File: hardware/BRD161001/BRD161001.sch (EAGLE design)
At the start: 42 parts, among them CN1 XH, CN2 JST XH, CN3 30306-6002HB, Q1 FDV301, Q2 DMP2035, Q3 FDV301, Q4 FDV301, U1 ATTINY44A-SSU, U2 TC4427AEOA, U3 TC4427AEOA, X1 32K768

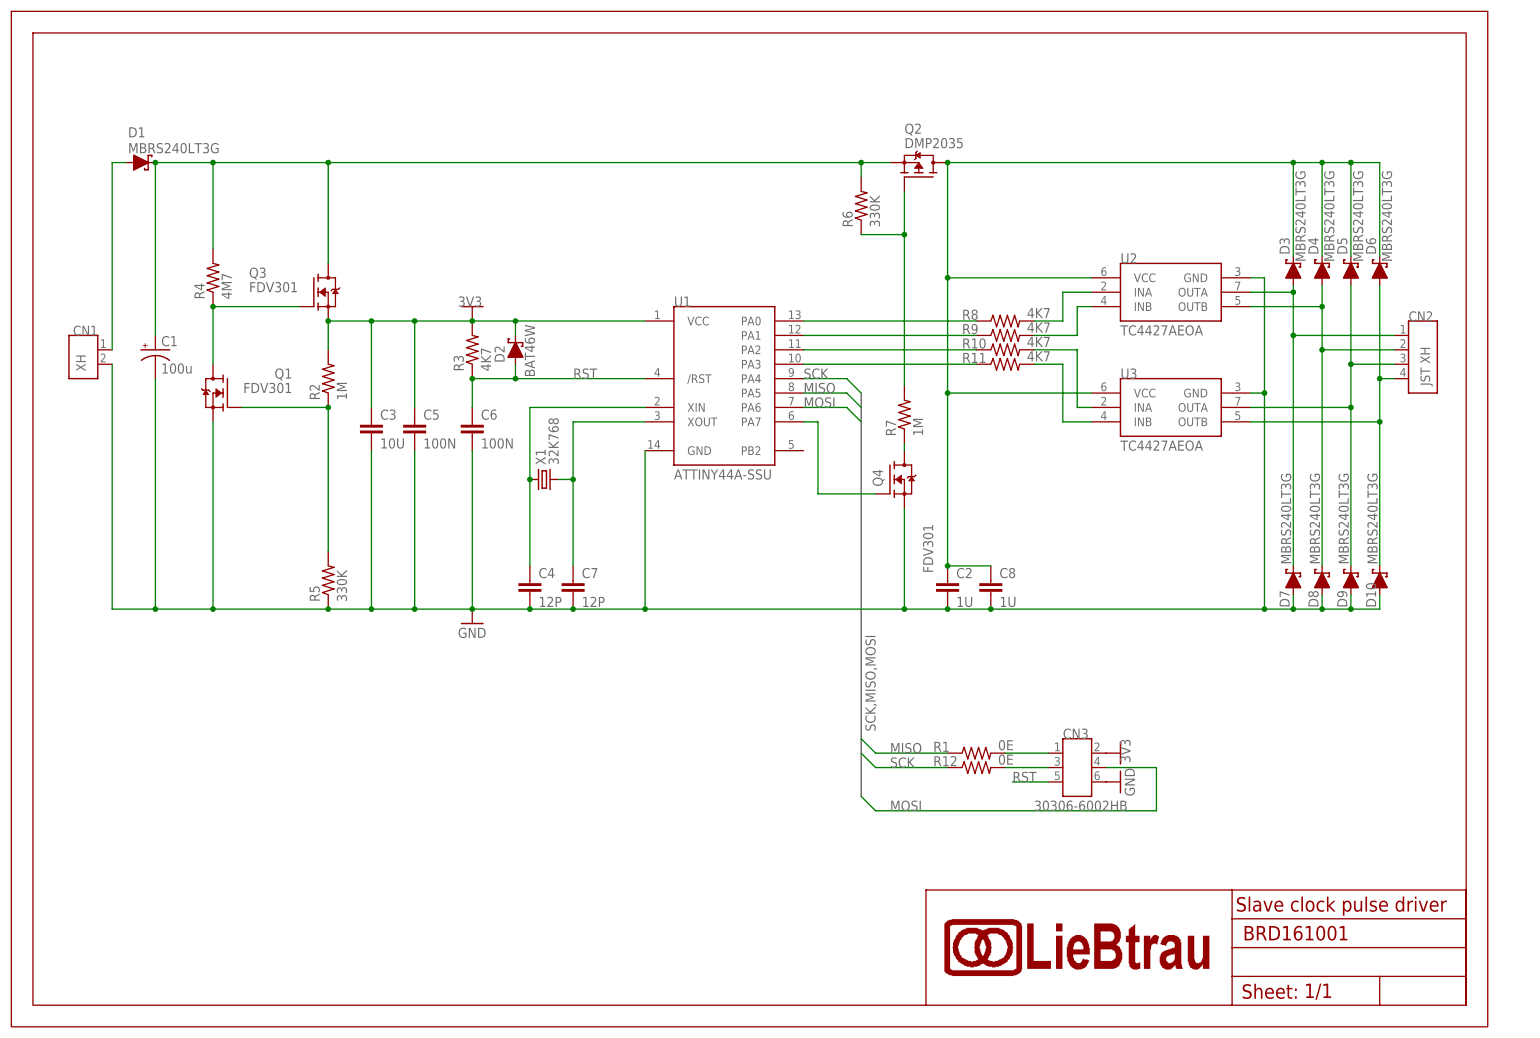
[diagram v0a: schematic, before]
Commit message: R1 of the hardware design
Signed-off-by: Christoph Tack <prog.send@gmail.com>
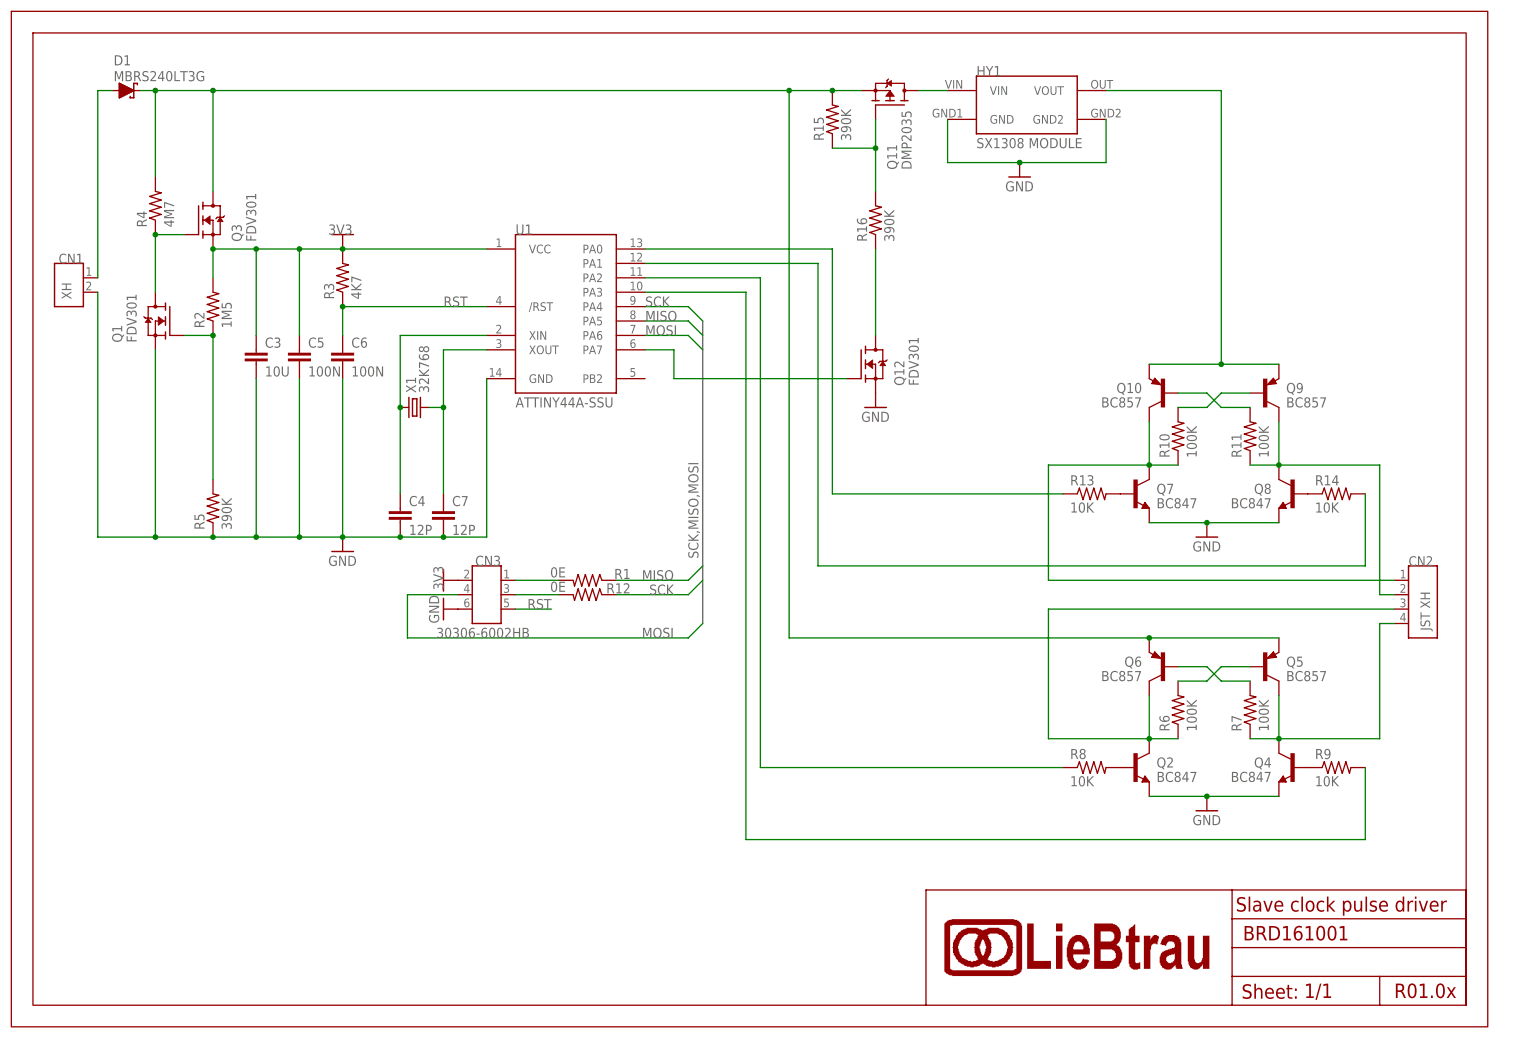
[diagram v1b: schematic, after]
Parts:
- removed C1: 100u, lieBtrau:CA_POL_100U_10X10
- removed C2, C8: 1U, lieBtrau:CA__1U_1206
- removed D10, D3, D4, D5, D6, D7, D8, D9: MBRS240LT3G, lieBtrau:DI_SCHOTTKYMBRS240DO-214AA
- removed D2: BAT46W, lieBtrau:DI_SCHOTTKYBAT46WSOD323
- removed U$1: FR_FRAME_A4, lieBtrau:FR_FRAME_A4
- removed U2, U3: TC4427AEOA, lieBtrau:IC_TC4427AEOA
- added FR1: FR_FRAME_A4A5, lieBtrau:FR_FRAME_A4A5
- added HY1: SX1308 MODULE, lieBtrau:HY_SX1308_SX1308__SX1308
- added Q10, Q5, Q6, Q9: BC857, lieBtrau:TR_PNP_BC857_SOT23
- added Q11: DMP2035, lieBtrau:TR_PMOSDMP2035_SOT23
- added Q12: FDV301, lieBtrau:TR_NMOSFDV301SOT23
- added Q7, Q8: BC847, lieBtrau:TR_NPN_BC847_SOT23
- added R13, R14: 10K, lieBtrau:RE_10K_1206
- added R15, R16: 390K, lieBtrau:RE_390K_1206
- Q2: value DMP2035 -> BC847; device lieBtrau:TR_PMOSDMP2035SOT23 -> lieBtrau:TR_NPN_BC847_SOT23
- Q4: value FDV301 -> BC847; device lieBtrau:TR_NMOSFDV301SOT23 -> lieBtrau:TR_NPN_BC847_SOT23
- R10, R11: value 4K7 -> 100K; device lieBtrau:RE__4K7_1206 -> lieBtrau:RE_100K_1206
- R2: value 1M -> 1M5; device lieBtrau:RE__1M_1206 -> lieBtrau:RE__1M5_1206
- R5: value 330K -> 390K; device lieBtrau:RE__330K_1206 -> lieBtrau:RE_390K_1206
- R6: value 330K -> 100K; device lieBtrau:RE__330K_1206 -> lieBtrau:RE_100K_1206
- R7: value 1M -> 100K; device lieBtrau:RE__1M_1206 -> lieBtrau:RE_100K_1206
- R8, R9: value 4K7 -> 10K; device lieBtrau:RE__4K7_1206 -> lieBtrau:RE_10K_1206
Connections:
- new net N$26: R13.1, U1.PA0
- new net N$27: Q12.G, U1.PA7
- new net N$28: Q12.D, R16.1
- new net N$29: HY1.VIN, Q11.D
- new net N$8: CN2.4, Q4.C, Q5.C, R7.1
- net 3V3: no longer D2.C
- net GND: now also HY1.GND, HY1.GND2, Q12.S, Q2.E, Q4.E, Q7.E, Q8.E; no longer C1.-, C2.2, C8.2, D10.A, D7.A, D8.A, D9.A, Q4.S, U2.GND, U3.GND
- net N$10: now also CN2.3, Q2.C, Q6.C, R6.1; no longer Q4.G, U1.PA7
- net N$11: now also Q2.B, R8.2; no longer C2.1, C8.1, D3.C, D4.C, D5.C, D6.C, Q2.D, U2.VCC, U3.VCC
- net N$12: now also Q4.B, R9.1; no longer R8.1, U1.PA0
- net N$13: now also HY1.VOUT, Q10.E, Q9.E; no longer R9.1, U1.PA1
- net N$14: now also R9.2, U1.PA3; no longer R10.1, U1.PA2
- net N$15: now also R8.1, U1.PA2; no longer R11.1, U1.PA3
- net N$16: now also Q9.B, R10.2; no longer R8.2, U2.INA
- net N$17: now also Q10.B, R11.2; no longer R9.2, U2.INB
- net N$18: now also Q7.B, R13.2; no longer R10.2, U3.INA
- net N$19: now also Q8.B, R14.1; no longer R11.2, U3.INB
- net N$2: now also D1.C, Q11.S, Q3.D, Q5.E, Q6.E, R15.2, R4.2; no longer Q2.G, R6.1, R7.2
- net N$20: now also R14.2, U1.PA1; no longer CN2.1, D3.A, D7.C, U2.OUTA
- net N$21: now also Q11.G, R15.1, R16.2; no longer CN2.2, D4.A, D8.C, U2.OUTB
- net N$22: now also CN2.2, Q8.C, Q9.C, R11.1; no longer CN2.3, D5.A, D9.C, U3.OUTA
- net N$23: now also CN2.1, Q10.C, Q7.C, R10.1; no longer CN2.4, D10.C, D6.A, U3.OUTB
- net N$3: now also Q5.B; no longer C1.+, D1.C, Q2.S, Q3.D, R4.2
- net N$5: now also Q6.B, R7.2; no longer Q4.D, R7.1
- net RST: no longer D2.A
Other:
- moved on the sheet: C3, C4, C5, C6, C7, CN1, CN2, CN3, D1, Q1, Q3, R1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

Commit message: working on R2 of PCB
Signed-off-by: Christoph Tack <prog.send@gmail.com>
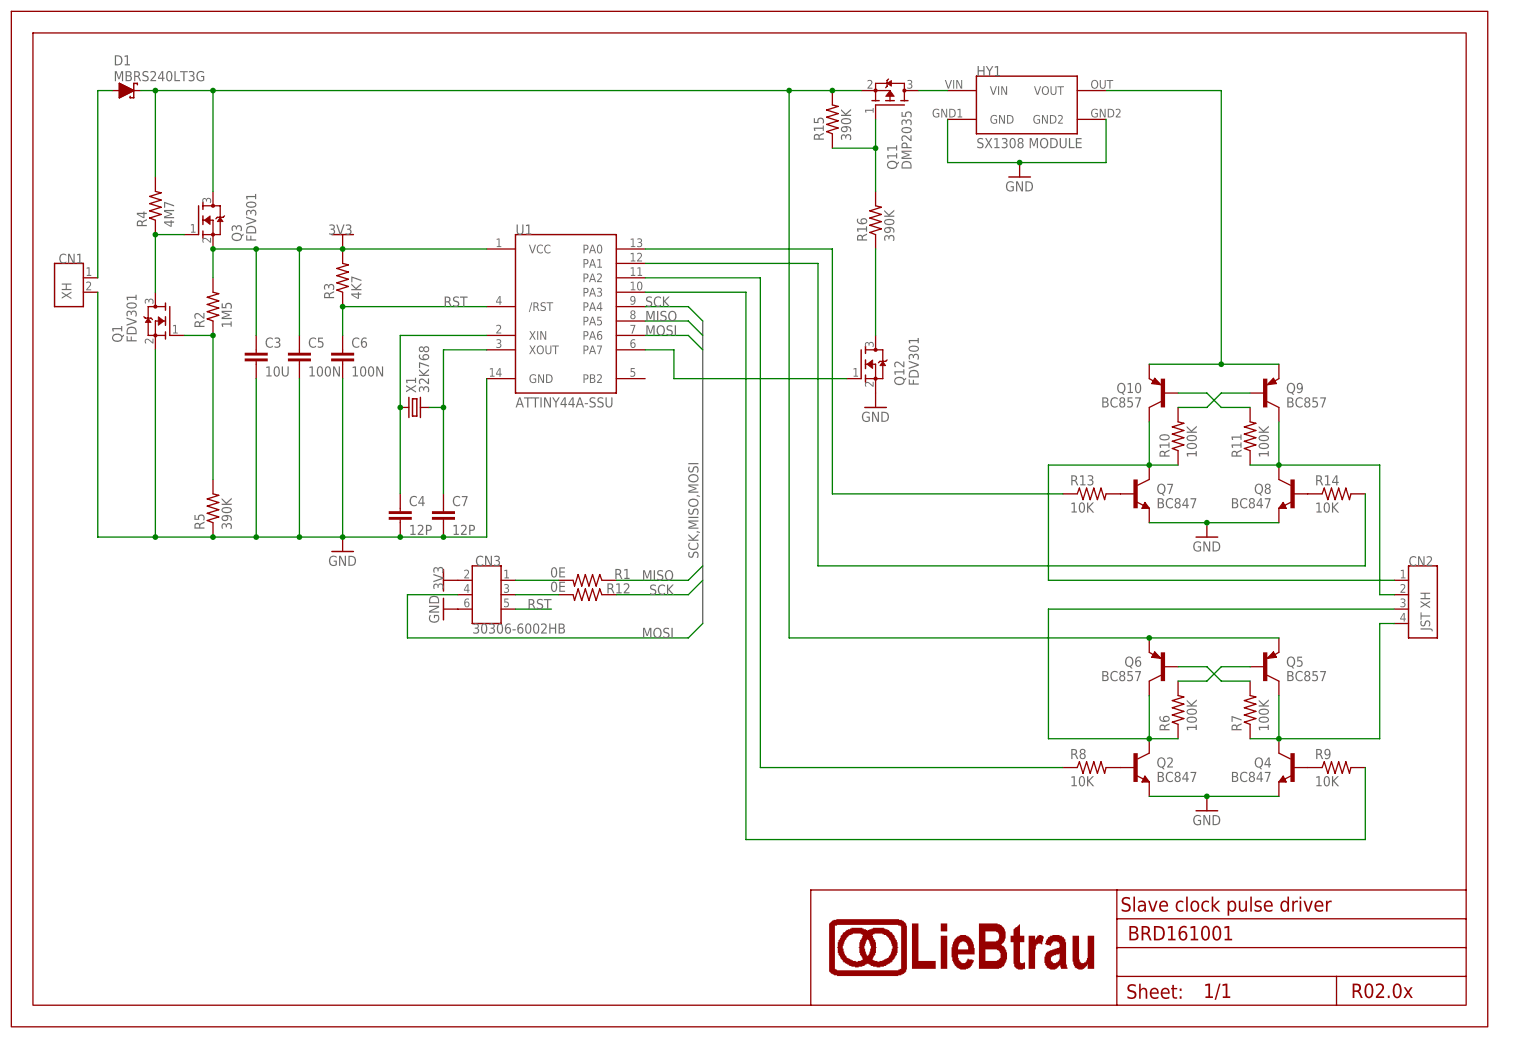
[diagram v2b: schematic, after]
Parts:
- CN1: device lieBtrau:CN_HDR1X2_180D_P25_JST_B2B-XH -> lieBtrau:CN_2P_JST_B2B-XH_JST_B2B-XH
- CN2: device lieBtrau:CN_HDR1X4_180D_P25_JST_B4B-XH -> lieBtrau:CN_4P_JST_B4B-XH_JST_B4B-XH
- CN3: device lieBtrau:CN_HDR2X3_180D_P25_3M -> lieBtrau:CN_2X3P_IDC_180D_P25_3M
- FR1: REV R01.0x -> R02.0x
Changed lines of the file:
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@@
 <parts>
 <part name="U1" library="lieBtrau" deviceset="IC_ATTINY44" device="SSU" value="ATTINY44A-SSU"/>
-<part name="CN1" library="lieBtrau" deviceset="CN_HDR1X2_180D_P25_JST_B2B-XH" device="" value="XH"/>
-<part name="CN2" library="lieBtrau" deviceset="CN_HDR1X4_180D_P25_JST_B4B-XH" device="" value="JST XH"/>
 <part name="D1" library="lieBtrau" deviceset="DI_SCHOTTKY" device="DO-214AA" technology="MBRS240" value="MBRS240LT3G"/>
 <part name="C3" library="lieBtrau" deviceset="CA_" device="1206" technology="_10U_" value="10U"/>
@@
 <part name="3V2" library="lieBtrau" deviceset="SY_3V3" device="" value="3V3"/>
 <part name="GND2" library="lieBtrau" deviceset="SY_GND" device="" value="GND"/>
-<part name="CN3" library="lieBtrau" deviceset="CN_HDR2X3_180D_P25_3M" device="" value="30306-6002HB"/>
 <part name="R2" library="lieBtrau" deviceset="RE_" device="1206" technology="_1M5_" value="1M5"/>
 <part name="R5" library="lieBtrau" deviceset="RE" device="1206" technology="_390K_" value="390K"/>
@@
 <part name="R16" library="lieBtrau" deviceset="RE" device="1206" technology="_390K_" value="390K"/>
 <part name="FR1" library="lieBtrau" deviceset="FR_FRAME_A4" device="A5">
-<attribute name="REV" value="R01.0x"/>
+<attribute name="REV" value="R02.0x"/>
 <attribute name="TITLE" value="Slave clock pulse driver"/>
 </part>
+<part name="CN1" library="lieBtrau" deviceset="CN_2P" device="JST_B2B-XH" technology="_JST_B2B-XH_" value="XH"/>
+<part name="CN2" library="lieBtrau" deviceset="CN_4P" device="JST_B4B-XH" technology="_JST_B4B-XH_" value="JST XH"/>
+<part name="CN3" library="lieBtrau" deviceset="CN_2X3P" device="180D_P25_3M" technology="_IDC_" value="30306-6002HB"/>
 </parts>
 <sheets>
@@
 <instances>
 <instance part="U1" gate="G$1" x="99.06" y="127"/>
-<instance part="CN1" gate="G$1" x="12.7" y="132.08" rot="MR0"/>
-<instance part="CN2" gate="G$1" x="246.38" y="76.2"/>
 <instance part="D1" gate="G$1" x="20.32" y="165.1" smashed="yes">
 <attribute name="NAME" x="18.034" y="169.545" size="1.778" layer="95"/>
@@
 <instance part="3V2" gate="G$1" x="76.2" y="78.74" rot="MR270"/>
 <instance part="GND2" gate="1" x="76.2" y="73.66" rot="MR90"/>
-<instance part="CN3" gate="G$1" x="83.82" y="76.2" smashed="yes" rot="MR0">
-<attribute name="VALUE" x="91.44" y="68.58" size="1.778" layer="96" rot="MR0"/>
-<attribute name="NAME" x="86.36" y="81.28" size="1.778" layer="95" rot="MR0"/>
-</instance>
 <instance part="R2" gate="G$1" x="35.56" y="127" rot="R90"/>
 <instance part="R5" gate="G$1" x="35.56" y="91.44" rot="R90"/>
@@
 <instance part="R16" gate="G$1" x="152.4" y="142.24" rot="R90"/>
 <instance part="FR1" gate="G$1" x="0" y="0"/>
+<instance part="CN1" gate="G$1" x="12.7" y="132.08" rot="MR0"/>
+<instance part="CN2" gate="G$1" x="246.38" y="76.2"/>
+<instance part="CN3" gate="G$1" x="83.82" y="76.2" smashed="yes" rot="MR0">
+<attribute name="VALUE" x="81.28" y="71.12" size="1.778" layer="96" rot="MR180"/>
+<attribute name="NAME" x="86.36" y="81.28" size="1.778" layer="95" rot="MR0"/>
+</instance>
 </instances>
 <busses>
@@
 <segment>
 <pinref part="D1" gate="G$1" pin="A"/>
-<pinref part="CN1" gate="G$1" pin="1"/>
 <wire x1="17.78" y1="165.1" x2="15.24" y2="165.1" width="0.1524" layer="91"/>
 <wire x1="15.24" y1="165.1" x2="15.24" y2="132.08" width="0.1524" layer="91"/>
+<pinref part="CN1" gate="G$1" pin="1"/>
 </segment>
 </net>
@@
 <net name="GND" class="0">
 <segment>
-<pinref part="CN1" gate="G$1" pin="2"/>
 <wire x1="15.24" y1="129.54" x2="15.24" y2="86.36" width="0.1524" layer="91"/>
 <pinref part="Q1" gate="G$1" pin="S"/>
@@
 <pinref part="R5" gate="G$1" pin="1"/>
 <junction x="35.56" y="86.36"/>
-</segment>
-<segment>
-<pinref part="GND2" gate="1" pin="GND"/>
-<pinref part="CN3" gate="G$1" pin="6"/>
+<pinref part="CN1" gate="G$1" pin="2"/>
 </segment>
 <segment>
@@
 <junction x="177.8" y="152.4"/>
 </segment>
+<segment>
+<pinref part="GND2" gate="1" pin="GND"/>
+<pinref part="CN3" gate="G$1" pin="6"/>
+</segment>
 </net>
 <net name="SCK" class="0">
@@
 <wire x1="223.52" y1="50.8" x2="241.3" y2="50.8" width="0.1524" layer="91"/>
 <wire x1="241.3" y1="50.8" x2="241.3" y2="71.12" width="0.1524" layer="91"/>
+<wire x1="241.3" y1="71.12" x2="243.84" y2="71.12" width="0.1524" layer="91"/>
 <pinref part="CN2" gate="G$1" pin="4"/>
-<wire x1="241.3" y1="71.12" x2="243.84" y2="71.12" width="0.1524" layer="91"/>
 </segment>
 </net>
@@
 <wire x1="223.52" y1="99.06" x2="241.3" y2="99.06" width="0.1524" layer="91"/>
 <wire x1="241.3" y1="76.2" x2="241.3" y2="99.06" width="0.1524" layer="91"/>
+<wire x1="243.84" y1="76.2" x2="241.3" y2="76.2" width="0.1524" layer="91"/>
 <pinref part="CN2" gate="G$1" pin="2"/>
-<wire x1="243.84" y1="76.2" x2="241.3" y2="76.2" width="0.1524" layer="91"/>
 </segment>
 </net>
@@
 <wire x1="182.88" y1="99.06" x2="200.66" y2="99.06" width="0.1524" layer="91"/>
 <wire x1="182.88" y1="99.06" x2="182.88" y2="78.74" width="0.1524" layer="91"/>
+<wire x1="243.84" y1="78.74" x2="182.88" y2="78.74" width="0.1524" layer="91"/>
 <pinref part="CN2" gate="G$1" pin="1"/>
-<wire x1="243.84" y1="78.74" x2="182.88" y2="78.74" width="0.1524" layer="91"/>
 </segment>
 </net>
@@
 <wire x1="182.88" y1="50.8" x2="200.66" y2="50.8" width="0.1524" layer="91"/>
 <wire x1="182.88" y1="73.66" x2="182.88" y2="50.8" width="0.1524" layer="91"/>
+<wire x1="243.84" y1="73.66" x2="182.88" y2="73.66" width="0.1524" layer="91"/>
 <pinref part="CN2" gate="G$1" pin="3"/>
-<wire x1="243.84" y1="73.66" x2="182.88" y2="73.66" width="0.1524" layer="91"/>
-</segment>
-</net>
+</segment>
+</net>
